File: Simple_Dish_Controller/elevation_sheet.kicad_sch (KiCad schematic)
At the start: 20 parts, among them J2 1-Pin Terminal Block, J7 RJ45 port shielded, RA, TH, J8 RJ45 port shielded, RA, TH, Q1 PZT2222A, Q2 PZT2222A, SW2 SW_SPDT_312, U2 74LS08, U3 74LS32, U4 NE555PS

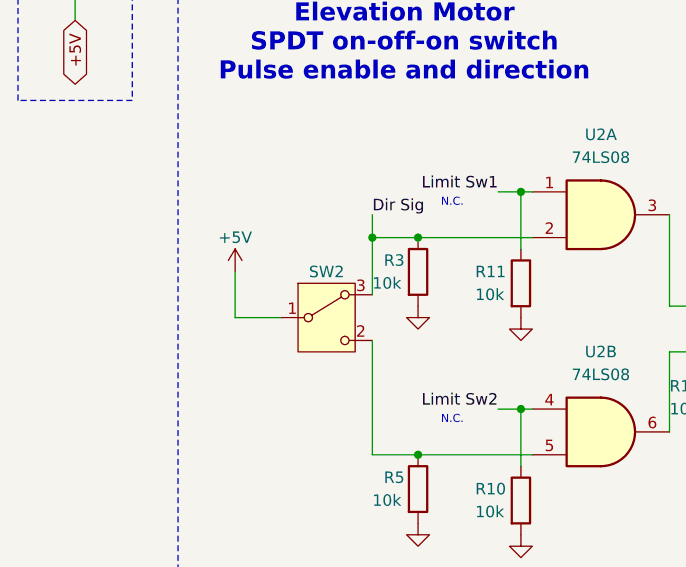
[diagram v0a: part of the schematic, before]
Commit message: Still creating parts libraries
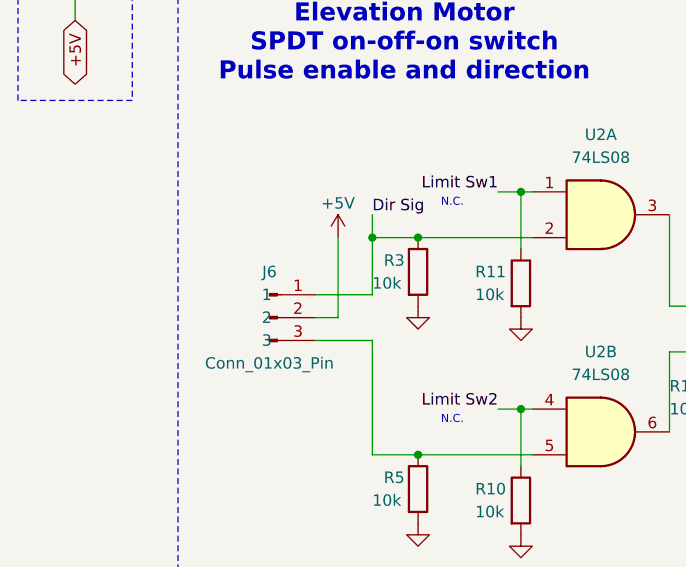
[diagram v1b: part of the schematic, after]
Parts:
- removed SW2: SW_SPDT_312, SPDT-90-Deg-On-Off-On:B18JH, symbol Switch:SW_SPDT_312
- added J6: Conn_01x03_Pin, DishFootprints:PinHeader_1x03_P2.54mm_Vertical, symbol DishSymbols:Conn_01x03_Pin
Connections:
- net +5V: now also J6.2
- net Dir Sig: now also J6.1
- net at R5.1, U2.5: now also J6.3
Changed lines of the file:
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@@
+	(wire
+		(pts
+			(xy 54.61 58.42) (xy 54.61 67.31)
+		)
+		(stroke
+			(width 0)
+			(type default)
+		)
+	)
 	(wire
 		(pts
@@
 	(wire
 		(pts
+			(xy 52.07 67.31) (xy 54.61 67.31)
+		)
+		(stroke
+			(width 0)
+			(type default)
+		)
+	)
+	(wire
+		(pts
 			(xy 228.6 53.34) (xy 236.22 53.34)
 		)
@@
 	(wire
 		(pts
-			(xy 48.26 67.31) (xy 43.18 67.31)
-		)
-		(stroke
-			(width 0)
-			(type default)
-		)
-	)
-	(wire
-		(pts
 			(xy 96.52 66.04) (xy 104.14 66.04)
 		)
@@
 	(wire
 		(pts
+			(xy 52.07 69.85) (xy 58.42 69.85)
+		)
+		(stroke
+			(width 0)
+			(type default)
+		)
+	)
+	(wire
+		(pts
 			(xy 195.58 50.8) (xy 195.58 52.07)
 		)
@@
 	(wire
 		(pts
+			(xy 52.07 64.77) (xy 58.42 64.77)
+		)
+		(stroke
+			(width 0)
+			(type default)
+		)
+	)
+	(wire
+		(pts
 			(xy 232.41 82.55) (xy 238.76 82.55)
 		)
@@
 		(pts
 			(xy 214.63 137.16) (xy 214.63 139.7)
-		)
-		(stroke
-			(width 0)
-			(type default)
-		)
-	)
-	(wire
-		(pts
-			(xy 43.18 67.31) (xy 43.18 62.23)
 		)
 		(stroke
@@
 	(symbol
 		(lib_id "power:+5V")
-		(at 43.18 62.23 0)
+		(at 54.61 58.42 0)
 		(unit 1)
 		(exclude_from_sim no)
@@
 		(dnp no)
 		(property "Reference" "#PWR09"
-			(at 43.18 66.04 0)
+			(at 54.61 62.23 0)
 			(effects
 				(font
@@
 		)
 		(property "Value" "+5V"
-			(at 43.18 58.42 0)
+			(at 54.61 54.61 0)
 			(effects
 				(font
@@
 		)
 		(property "Footprint" ""
-			(at 43.18 62.23 0)
+			(at 54.61 58.42 0)
 			(effects
 				(font
@@
 		)
 		(property "Datasheet" ""
-			(at 43.18 62.23 0)
+			(at 54.61 58.42 0)
 			(effects
 				(font
@@
 		)
 		(property "Description" "Power symbol creates a global label with name \"+5V\""
-			(at 43.18 62.23 0)
+			(at 54.61 58.42 0)
 			(effects
 				(font
@@
 	)
 	(symbol
+		(lib_id "DishSymbols:Conn_01x03_Pin")
+		(at 46.99 67.31 0)
+		(unit 1)
+		(exclude_from_sim no)
+		(in_bom yes)
+		(on_board yes)
+		(dnp no)
+		(property "Reference" "J6"
+			(at 46.99 62.23 0)
+			(effects
+				(font
+					(size 1.27 1.27)
+				)
+			)
+		)
+		(property "Value" "Conn_01x03_Pin"
+			(at 46.99 72.39 0)
+			(effects
+				(font
+					(size 1.27 1.27)
+				)
+			)
+		)
+		(property "Footprint" "DishFootprints:PinHeader_1x03_P2.54mm_Vertical"
+			(at 46.99 67.31 0)
+			(effects
+				(font
+					(size 1.27 1.27)
+				)
+				(hide yes)
+			)
+		)
+		(property "Datasheet" "~https://app.adam-tech.com/products/download/data_sheet/201605/ph1-xx-ua-data-sheet.pdf"
+			(at 46.99 67.31 0)
+			(effects
+				(font
+					(size 1.27 1.27)
+				)
+				(hide yes)
+			)
+		)
+		(property "Description" "Connector Header Through Hole 3 position 0.100\" (2.54mm)"
+			(at 46.99 67.31 0)
+			(effects
+				(font
+					(size 1.27 1.27)
+				)
+				(hide yes)
+			)
+		)
+		(property "Package" "-"
+			(at 46.99 67.31 0)
+			(effects
+				(font
+					(size 1 1)
+				)
+				(hide yes)
+			)
+		)
+		(property "MF" "Adam Tech"
+			(at 46.99 67.31 0)
+			(effects
+				(font
+					(size 1 1)
+				)
+				(hide yes)
+			)
+		)
+		(property "MPN" "PH1-03-UA"
+			(at 46.99 67.31 0)
+			(effects
+				(font
+					(size 1 1)
+				)
+				(hide yes)
+			)
+		)
+		(property "DIS" "Digikey"
+			(at 46.99 67.31 0)
+			(effects
+				(font
+					(size 1 1)
+				)
+				(hide yes)
+			)
+		)
+		(property "DPN" "2057-PH1-03-UA-ND"
+			(at 46.99 67.31 0)
+			(effects
+				(font
+					(size 1 1)
+				)
+				(hide yes)
+			)
+		)
+		(property "Purchase_URL" "https://www.digikey.com/en/products/detail/adam-tech/PH1-03-UA/9830289"
+			(at 46.99 67.31 0)
+			(effects
+				(font
+					(size 1 1)
+				)
+				(hide yes)
+			)
+		)
+		(property "Price" "0.04"
+			(at 46.99 67.31 0)
+			(effects
+				(font
+					(size 1 1)
+				)
+				(hide yes)
+			)
+		)
+		(property "Note" ""
+			(at 46.99 67.31 0)
+			(effects
+				(font
+					(size 1 1)
+				)
+				(hide yes)
+			)
+		)
+		(pin "3"
+		)
+		(pin "1"
+		)
+		(pin "2"
+		)
+		(instances
+			(project ""
+				(path "/8648ccd3-30ce-4b98-baff-aeab56a7c9f5/a4809f50-064d-4cb7-b1f7-56bf09fb0ea4"
+					(reference "J6")
+					(unit 1)
+				)
+			)
+		)
+	)
+	(symbol
 		(lib_id "power:GND")
 		(at 69.85 172.72 0)
@@
 					(unit 1)
 				)
-			)
-		)
-	)
-	(symbol
-		(lib_id "Switch:SW_SPDT_312")
-		(at 53.34 67.31 0)
-		(unit 1)
-		(exclude_from_sim no)
-		(in_bom yes)
-		(on_board yes)
-		(dnp no)
-		(property "Reference" "SW2"
-			(at 53.34 62.23 0)
-			(effects
-				(font
-					(size 1.27 1.27)
-				)
-			)
-		)
-		(property "Value" "SW_SPDT_312"
-			(at 53.34 60.96 0)
-			(effects
-				(font
-					(size 1.27 1.27)
-				)
-				(hide yes)
-			)
-		)
-		(property "Footprint" "SPDT-90-Deg-On-Off-On:B18JH"
-			(at 53.34 77.47 0)
-			(effects
-				(font
-					(size 1.27 1.27)
-				)
-				(hide yes)
-			)
-		)
-		(property "Datasheet" "~"
-			(at 53.34 74.93 0)
-			(effects
-				(font
-					(size 1.27 1.27)
-				)
-				(hide yes)
-			)
-		)
-		(property "Description" "Switch, single pole double throw"
-			(at 53.34 67.31 0)
-			(effects
-				(font
-					(size 1.27 1.27)
-				)
-				(hide yes)
-			)
-		)
-		(property "LCSC Part" ""
-			(at 53.34 67.31 0)
-			(effects
-				(font
-					(size 1.27 1.27)
-				)
-			)
-		)
-		(pin "2"
-		)
-		(pin "1"
-		)
-		(pin "3"
-		)
-		(instances
-			(project "simple_dish_manual_controller"
-				(path "/8648ccd3-30ce-4b98-baff-aeab56a7c9f5/a4809f50-064d-4cb7-b1f7-56bf09fb0ea4"
-					(reference "SW2")
-					(unit 1)
-				)
